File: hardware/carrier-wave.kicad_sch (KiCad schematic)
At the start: 4 parts, among them U2 OPA695, U3 THS3491, U4 AD9834, U7 TS5A3159ADCK

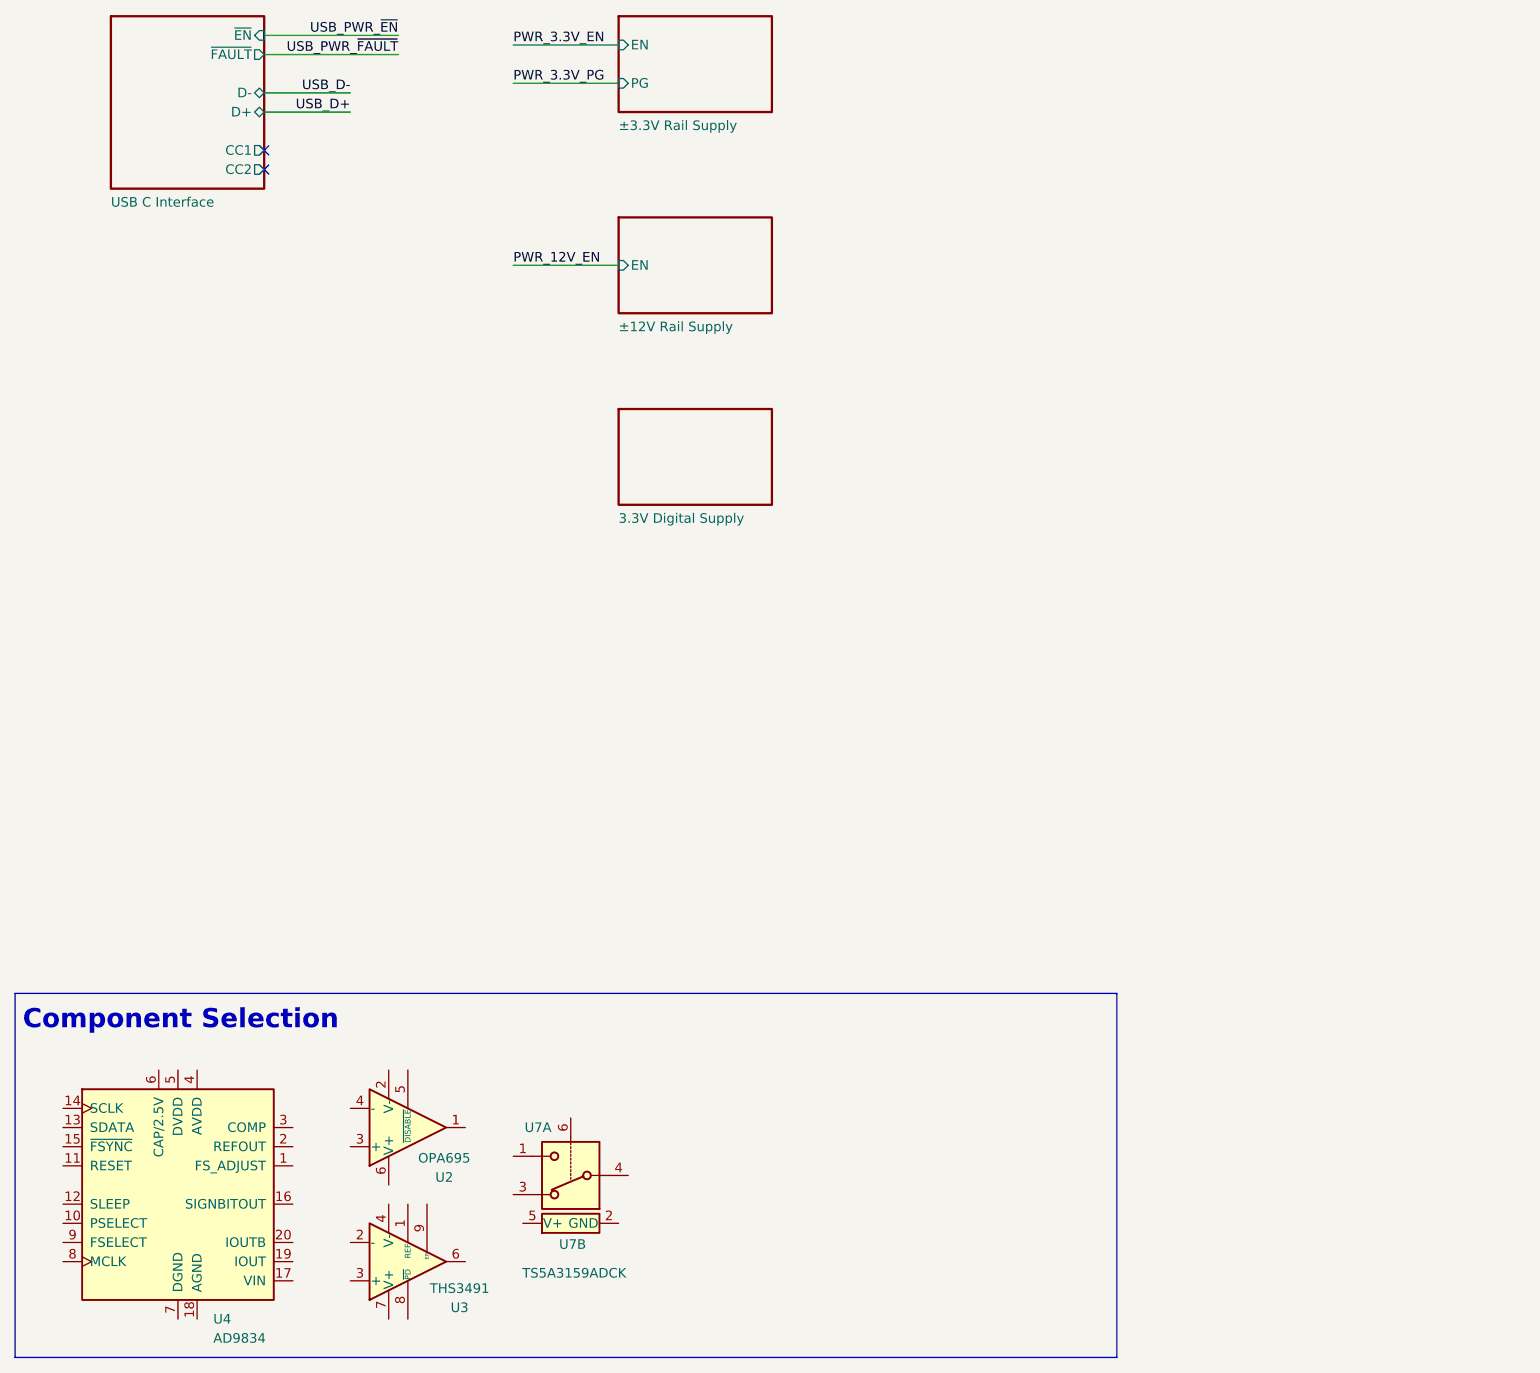
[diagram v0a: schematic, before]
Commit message: Begin MCU
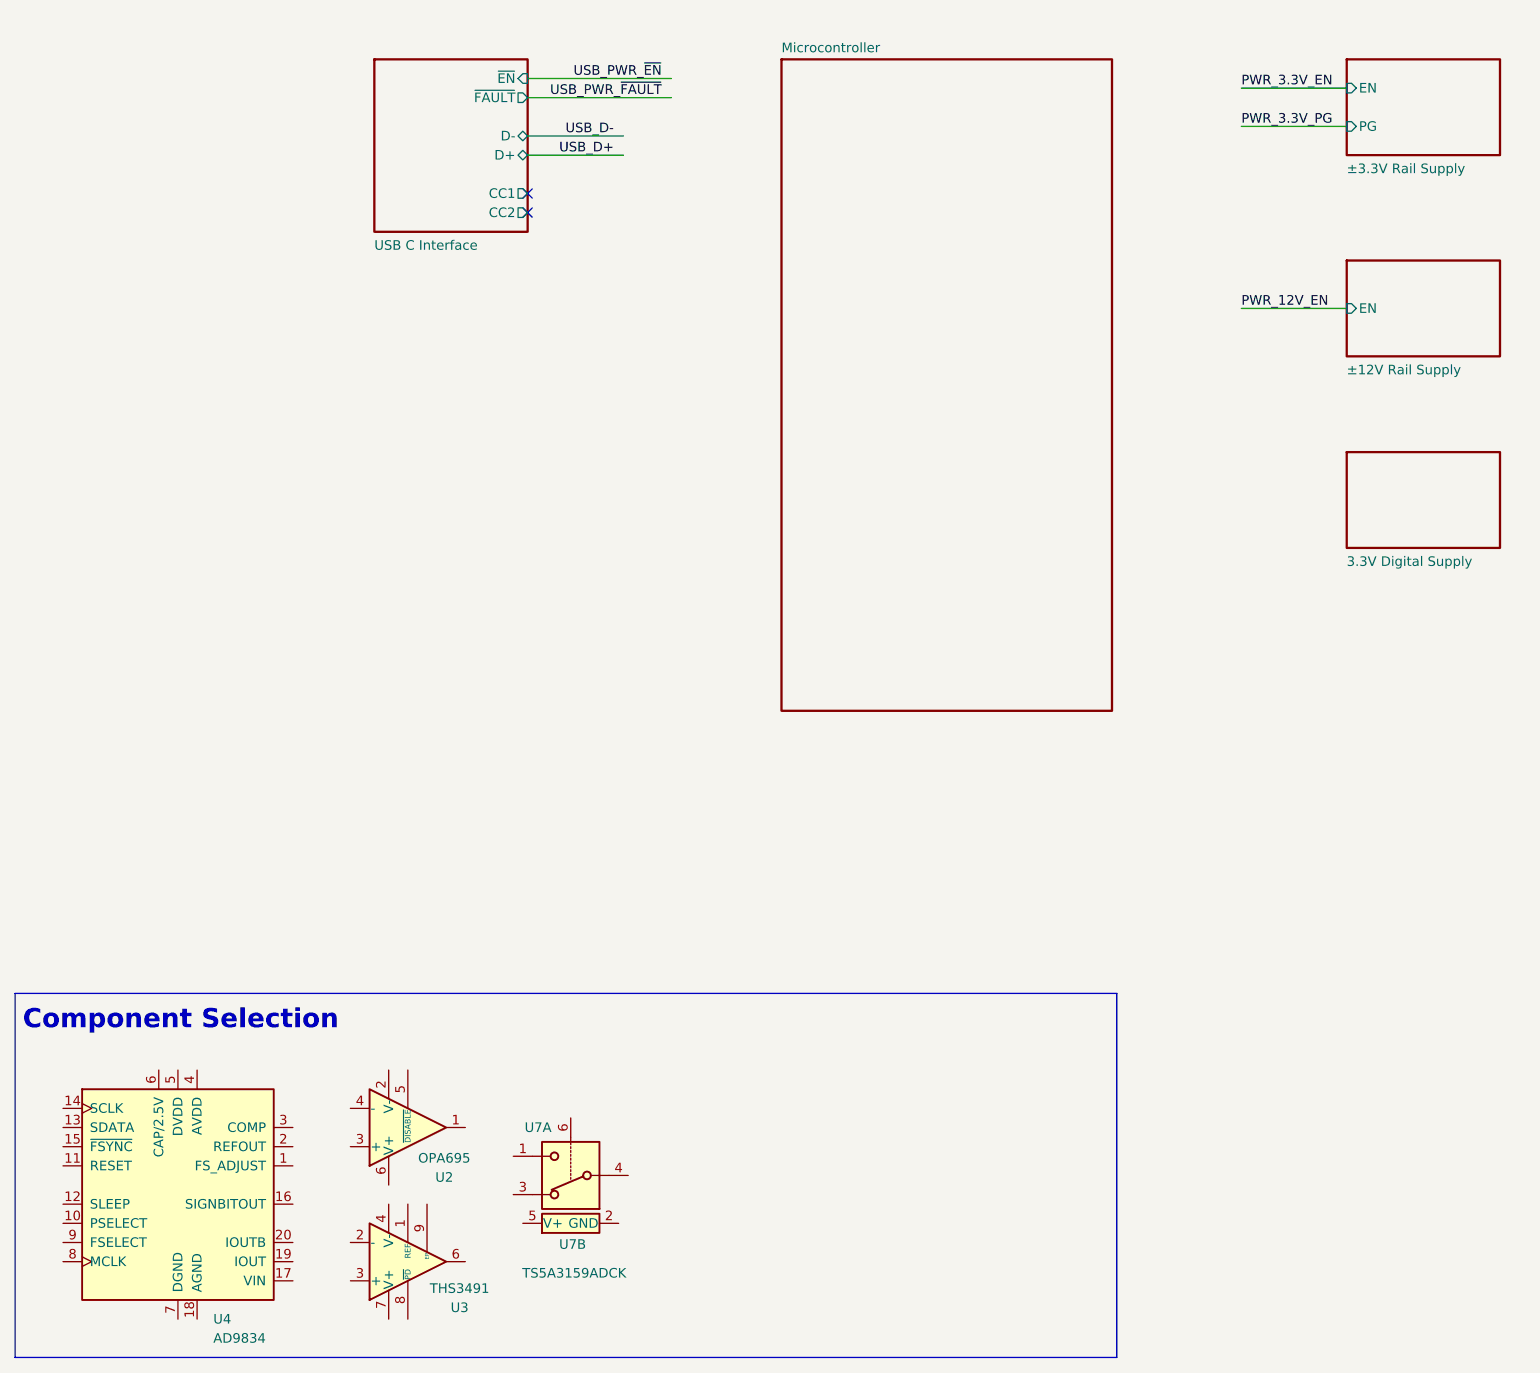
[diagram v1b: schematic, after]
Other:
- added sheet Microcontroller (microcontroller.kicad_sch)
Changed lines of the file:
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@@
 	)
 	(no_connect
-		(at 45.72 45.72)
+		(at 80.645 51.435)
 	)
 	(no_connect
-		(at 45.72 43.18)
+		(at 80.645 48.895)
 	)
 	(wire
 		(pts
-			(xy 92.71 29.21) (xy 78.74 29.21)
+			(xy 189.23 34.925) (xy 175.26 34.925)
 		)
 		(stroke
@@
 	(wire
 		(pts
-			(xy 78.74 34.29) (xy 92.71 34.29)
+			(xy 175.26 40.005) (xy 189.23 40.005)
 		)
 		(stroke
@@
 	(wire
 		(pts
-			(xy 45.72 35.56) (xy 57.15 35.56)
+			(xy 80.645 41.275) (xy 93.345 41.275)
 		)
 		(stroke
@@
 	(wire
 		(pts
-			(xy 78.74 58.42) (xy 92.71 58.42)
+			(xy 175.26 64.135) (xy 189.23 64.135)
 		)
 		(stroke
@@
 	(wire
 		(pts
-			(xy 45.72 27.94) (xy 63.5 27.94)
+			(xy 80.645 33.655) (xy 99.695 33.655)
 		)
 		(stroke
@@
 	(wire
 		(pts
-			(xy 45.72 38.1) (xy 57.15 38.1)
+			(xy 80.645 43.815) (xy 93.345 43.815)
 		)
 		(stroke
@@
 	(wire
 		(pts
-			(xy 45.72 30.48) (xy 63.5 30.48)
+			(xy 80.645 36.195) (xy 99.695 36.195)
 		)
 		(stroke
@@
 	)
 	(label "USB_PWR_~{EN}"
-		(at 63.5 27.94 180)
+		(at 98.425 33.655 180)
 		(effects
 			(font
@@
 	)
 	(label "USB_D+"
-		(at 57.15 38.1 180)
+		(at 92.075 43.815 180)
 		(effects
 			(font
@@
 	)
 	(label "PWR_3.3V_EN"
-		(at 78.74 29.21 0)
+		(at 175.26 34.925 0)
 		(effects
 			(font
@@
 	)
 	(label "PWR_3.3V_PG"
-		(at 78.74 34.29 0)
+		(at 175.26 40.005 0)
 		(effects
 			(font
@@
 	)
 	(label "USB_D-"
-		(at 57.15 35.56 180)
+		(at 92.075 41.275 180)
 		(effects
 			(font
@@
 	)
 	(label "USB_PWR_~{FAULT}"
-		(at 63.5 30.48 180)
+		(at 98.425 36.195 180)
 		(effects
 			(font
@@
 	)
 	(label "PWR_12V_EN"
-		(at 78.74 58.42 0)
+		(at 175.26 64.135 0)
 		(effects
 			(font
@@
 	)
 	(sheet
-		(at 92.71 52.07)
+		(at 189.23 57.785)
 		(size 20.32 12.7)
 		(exclude_from_sim no)
@@
 		)
 		(property "Sheetname" "±12V Rail Supply"
-			(at 92.71 67.31 0)
+			(at 189.23 73.025 0)
 			(show_name no)
 			(do_not_autoplace no)
@@
 		)
 		(property "Sheetfile" "12V_boost_converter.kicad_sch"
-			(at 92.71 65.3546 0)
+			(at 189.23 71.0696 0)
 			(hide yes)
 			(show_name no)
@@
 		)
 		(property "Component" "TPS65131RGE / LM2940 & LM2990"
-			(at 110.49 50.8 0)
+			(at 207.01 56.515 0)
 			(hide yes)
 			(show_name no)
@@
 		)
 		(pin "EN" input
-			(at 92.71 58.42 180)
+			(at 189.23 64.135 180)
 			(effects
 				(font
@@
 	)
 	(sheet
-		(at 92.71 77.47)
+		(at 189.23 83.185)
 		(size 20.32 12.7)
 		(exclude_from_sim no)
@@
 		)
 		(property "Sheetname" "3.3V Digital Supply"
-			(at 92.71 92.71 0)
+			(at 189.23 98.425 0)
 			(show_name no)
 			(do_not_autoplace no)
@@
 		)
 		(property "Sheetfile" "3V_digital_supply.kicad_sch"
-			(at 92.71 90.8308 0)
+			(at 189.23 96.5458 0)
 			(hide yes)
 			(show_name no)
@@
 	)
 	(sheet
-		(at 92.71 25.4)
+		(at 189.23 31.115)
 		(size 20.32 12.7)
 		(exclude_from_sim no)
@@
 		)
 		(property "Sheetname" "±3.3V Rail Supply"
-			(at 92.71 40.64 0)
+			(at 189.23 46.355 0)
 			(show_name no)
 			(do_not_autoplace no)
@@
 		)
 		(property "Sheetfile" "charge_pump_ldo.kicad_sch"
-			(at 92.71 38.6846 0)
+			(at 189.23 44.3996 0)
 			(hide yes)
 			(show_name no)
@@
 		)
 		(pin "EN" input
-			(at 92.71 29.21 180)
+			(at 189.23 34.925 180)
 			(effects
 				(font
@@
 		)
 		(pin "PG" input
-			(at 92.71 34.29 180)
+			(at 189.23 40.005 180)
 			(effects
 				(font
@@
 	)
 	(sheet
-		(at 25.4 25.4)
+		(at 60.325 31.115)
 		(size 20.32 22.86)
 		(exclude_from_sim no)
@@
 		)
 		(property "Sheetname" "USB C Interface"
-			(at 25.4 50.8 0)
+			(at 60.325 56.515 0)
 			(show_name no)
 			(do_not_autoplace no)
@@
 		)
 		(property "Sheetfile" "usb_interface.kicad_sch"
-			(at 25.4 38.7608 0)
+			(at 60.325 44.4758 0)
 			(hide yes)
 			(show_name no)
@@
 		)
 		(pin "CC1" output
-			(at 45.72 43.18 0)
+			(at 80.645 48.895 0)
 			(effects
 				(font
@@
 		)
 		(pin "CC2" output
-			(at 45.72 45.72 0)
+			(at 80.645 51.435 0)
 			(effects
 				(font
@@
 		)
 		(pin "D+" bidirectional
-			(at 45.72 38.1 0)
+			(at 80.645 43.815 0)
 			(effects
 				(font
@@
 		)
 		(pin "D-" bidirectional
-			(at 45.72 35.56 0)
+			(at 80.645 41.275 0)
 			(effects
 				(font
@@
 		)
 		(pin "~{EN}" input
-			(at 45.72 27.94 0)
+			(at 80.645 33.655 0)
 			(effects
 				(font
@@
 		)
 		(pin "~{FAULT}" output
-			(at 45.72 30.48 0)
+			(at 80.645 36.195 0)
 			(effects
 				(font
@@
 				)
 			)
+		)
+	)
+	(sheet
+		(at 114.3 31.115)
+		(size 43.815 86.36)
+		(exclude_from_sim no)
+		(in_bom yes)
+		(on_board yes)
+		(dnp no)
+		(fields_autoplaced yes)
+		(stroke
+			(width 0.3048)
+			(type solid)
+		)
+		(fill
+			(color 255 229 191 1)
+		)
+		(property "Sheetname" "Microcontroller"
+			(at 114.3 30.3272 0)
+			(show_name no)
+			(do_not_autoplace no)
+			(effects
+				(font
+					(size 1.27 1.27)
+				)
+				(justify left bottom)
+			)
+		)
+		(property "Sheetfile" "microcontroller.kicad_sch"
+			(at 114.3 118.1358 0)
+			(hide yes)
+			(show_name no)
+			(do_not_autoplace no)
+			(effects
+				(font
+					(size 1.27 1.27)
+				)
+				(justify left top)
+			)
+		)
+		(instances
+			(project "carrier-wave"
+				(path "/dc900721-a2e3-4f11-b4f2-59bb3a47422e"
+					(page "5")
+				)
+			)
